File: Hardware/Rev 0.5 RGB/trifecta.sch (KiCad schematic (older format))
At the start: 284 parts, among them J1 USB2_C_Receptacle, SW1 SW_Push, SW2 Rotary_Encoder_Switch, SW3 Rotary_Encoder_Switch, SW4 Rotary_Encoder_Switch, U1 ATmega32U4-AU, U2 SRV05-4, Y1 16MHz

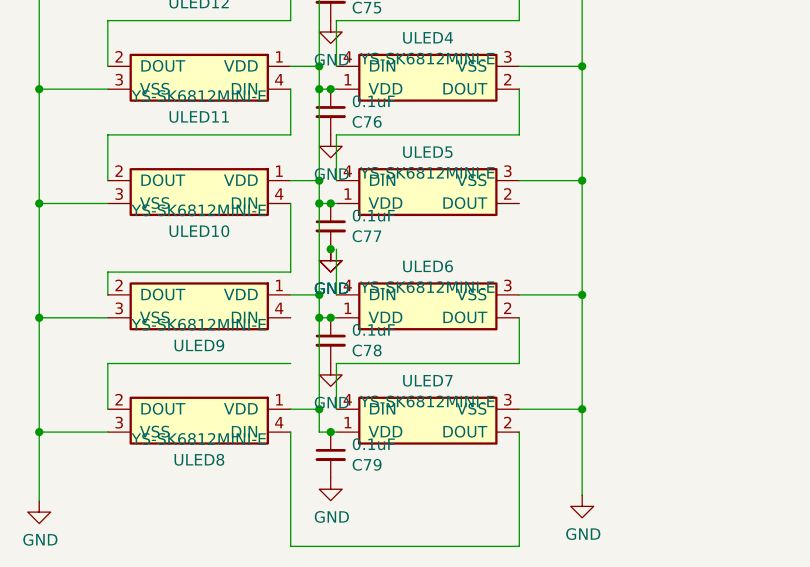
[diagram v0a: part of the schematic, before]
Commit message: 08/07
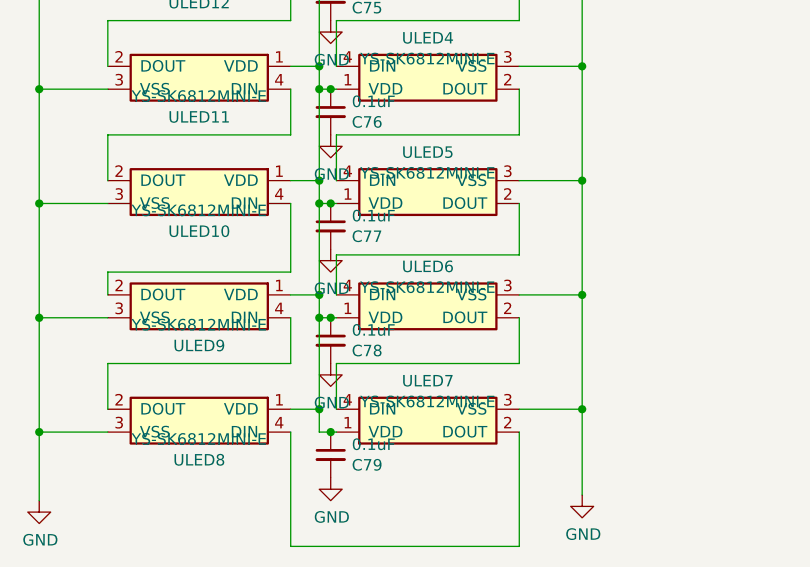
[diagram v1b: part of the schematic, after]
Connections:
- net at ULED5.2 (DOUT): now also ULED6.4 (DIN)
- net at ULED9.4 (DIN): now also ULED8.2 (DOUT)
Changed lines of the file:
@@
-$EndComp
-$Comp
-L power:GND #PWR0157
-U 1 1 5FB8AEBA
-P 25900 5275
-F 0 "#PWR0157" H 25900 5025 50  0001 C CNN
-F 1 "GND" H 25905 5102 50  0000 C CNN
-F 2 "" H 25900 5275 50  0001 C CNN
-F 3 "" H 25900 5275 50  0001 C CNN
-	1    25900 5275
-	1    0    0    -1
 $EndComp
 $Comp
@@
 	25900 6075 25850 6075
 Wire Wire Line
-	25925 5475 25925 5275
-Wire Wire Line
 	25925 5575 25900 5575
 Wire Wire Line
@@
 $EndComp
 Connection ~ 25850 5075
-Connection ~ 25900 5275
 Wire Wire Line
 	25925 2625 25925 2975
@@
 	-1   0    0    -1
 $EndComp
+Wire Wire Line
+	25925 5475 25925 5300
+Wire Wire Line
+	25925 5300 26725 5300
+Wire Wire Line
+	26725 5300 26725 5075
+Wire Wire Line
+	25725 5775 25725 5575
 $EndSCHEMATC

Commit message: LED37
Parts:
- K_15: footprint MX_Only:MXOnly-2U-NoLED -> MX_Only:MXOnly-2U-ReversedStabilizers-NoLED
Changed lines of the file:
@@
 F 0 "K_15" H 18275 8808 60  0000 C CNN
 F 1 "KEYSW" H 18275 8475 60  0001 C CNN
-F 2 "MX_Only:MXOnly-2U-NoLED" H 18275 8575 60  0001 C CNN
+F 2 "MX_Only:MXOnly-2U-ReversedStabilizers-NoLED" H 18275 8575 60  0001 C CNN
 F 3 "" H 18275 8575 60  0000 C CNN
 	1    18275 8575
